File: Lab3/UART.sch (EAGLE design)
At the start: 11 parts, among them IC1 74AC11138, IC2 LM358N, IC3 LM358D, U1 AD558

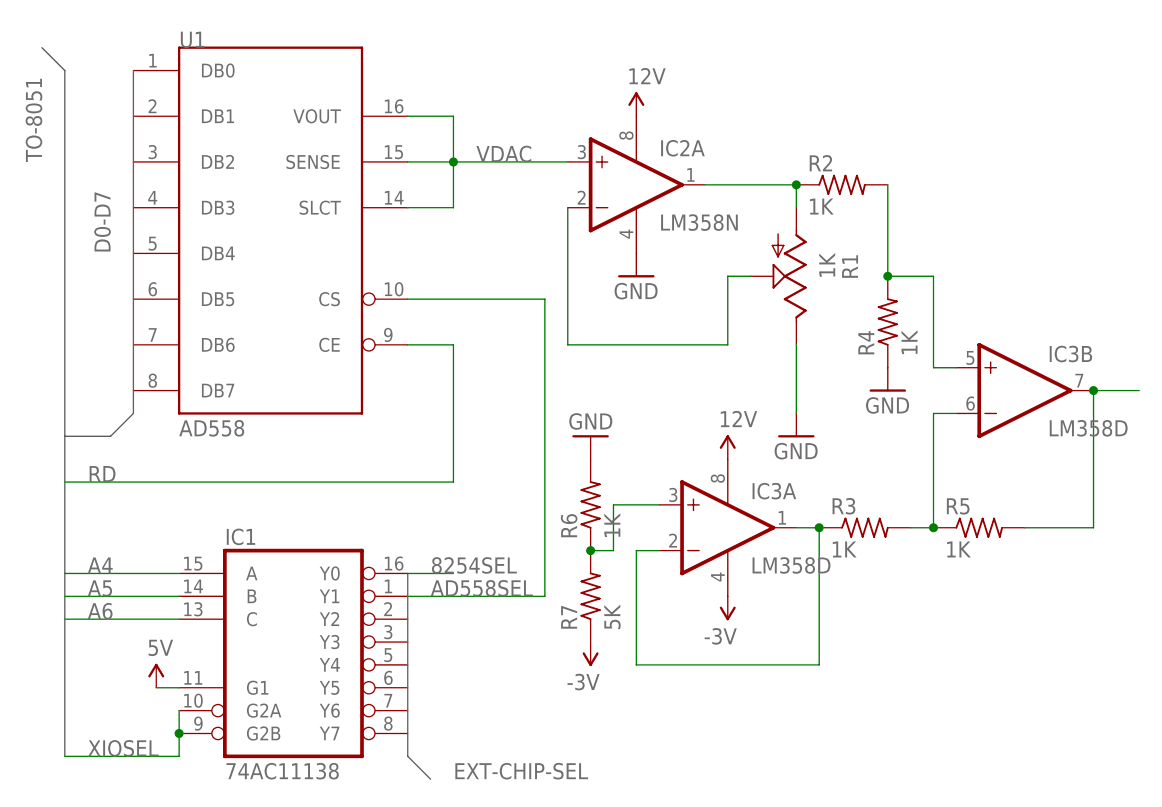
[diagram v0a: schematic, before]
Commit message: halfway through lab 4
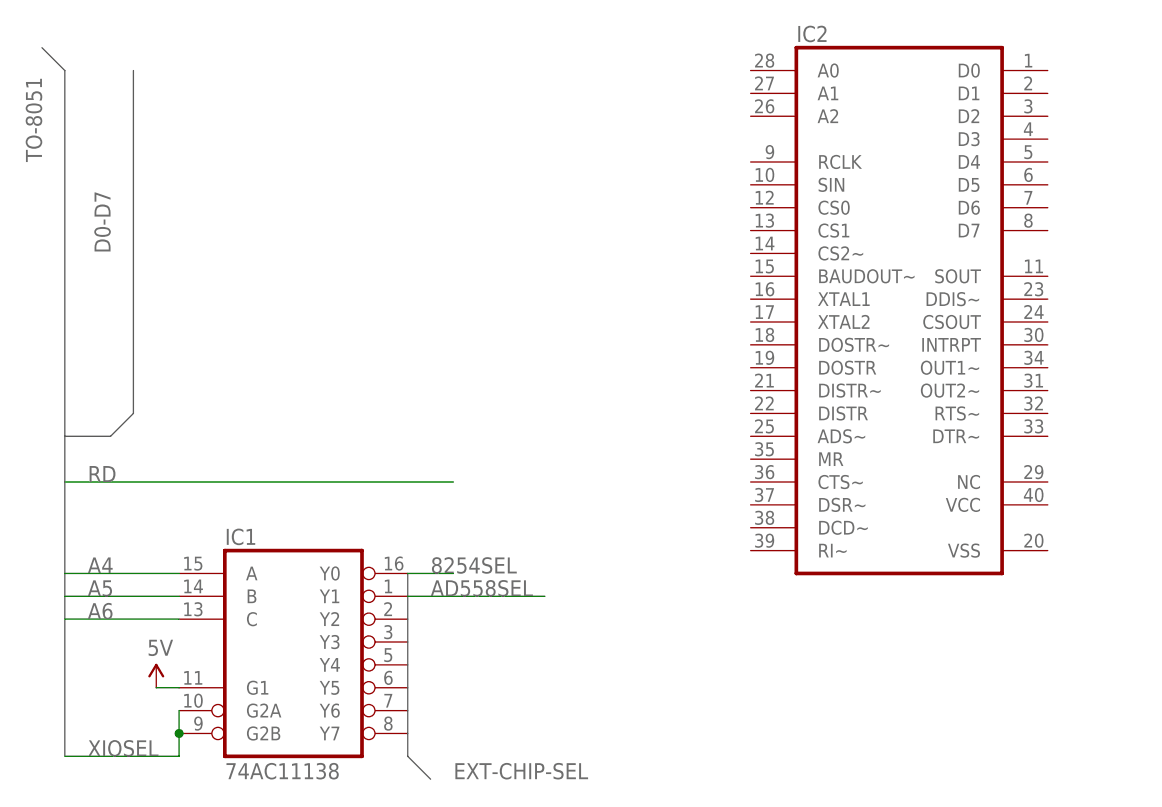
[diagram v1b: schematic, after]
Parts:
- removed IC3: LM358D, linear:LM358D
- removed R1: 1K, pot:TRIM_US-3223G
- removed R2, R3, R4, R5, R6: 1K, resistor:R-US_0204/2V
- removed R7: 5K, resistor:R-US_0204/2V
- removed U1: AD558, AD558:AD558
- IC2: value LM358N -> (none); device linear:LM358N -> exar:XR-16C450P
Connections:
- removed net GND: IC2P.V-, R1.E, R4.1, R6.2
- removed net N$1: IC2A.OUT, R1.A, R2.1
- removed net N$2: IC2A.-IN, R1.S
- removed net N$3: IC3A.-IN, IC3A.OUT, R3.1
- removed net N$4: IC3A.+IN, R6.1, R7.2
- removed net N$5: IC3B.+IN, R2.2, R4.2
- removed net N$6: IC3B.-IN, R3.2, R5.1
- removed net N$8: IC3B.OUT, R5.2
- removed net RD: U1AD558.CE
- removed net VDAC: IC2A.+IN, U1AD558.SENSE, U1AD558.SLCT, U1AD558.VOUT
- net 5V: no longer IC2P.V+, IC3P.V+, IC3P.V-, R7.1
- net AD558SEL: no longer U1AD558.CS
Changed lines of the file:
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@@
 <parts>
 <part name="IC1" library="74ac-logic" deviceset="74AC11138" device=""/>
-<part name="U1" library="AD558" deviceset="AD558" device=""/>
-<part name="IC2" library="linear" deviceset="LM358" device="N"/>
-<part name="R1" library="pot" deviceset="TRIM_US-" device="3223G" value="1K"/>
-<part name="GND1" library="SparkFun-Aesthetics" deviceset="GND" device=""/>
-<part name="SUPPLY1" library="SparkFun-Aesthetics" deviceset="5V" device="" value="12V"/>
 <part name="SUPPLY2" library="SparkFun-Aesthetics" deviceset="5V" device=""/>
-<part name="GND2" library="SparkFun-Aesthetics" deviceset="GND" device=""/>
-<part name="IC3" library="linear" deviceset="LM358" device="D"/>
-<part name="R2" library="resistor" deviceset="R-US_" device="0204/2V" value="1K"/>
-<part name="R3" library="resistor" deviceset="R-US_" device="0204/2V" value="1K"/>
-<part name="R4" library="resistor" deviceset="R-US_" device="0204/2V" value="1K"/>
-<part name="R5" library="resistor" deviceset="R-US_" device="0204/2V" value="1K"/>
-<part name="R6" library="resistor" deviceset="R-US_" device="0204/2V" value="1K"/>
-<part name="R7" library="resistor" deviceset="R-US_" device="0204/2V" value="5K"/>
-<part name="SUPPLY3" library="SparkFun-Aesthetics" deviceset="5V" device="" value="-3V"/>
-<part name="SUPPLY4" library="SparkFun-Aesthetics" deviceset="5V" device="" value="12V"/>
-<part name="SUPPLY5" library="SparkFun-Aesthetics" deviceset="5V" device="" value="-3V"/>
-<part name="GND3" library="SparkFun-Aesthetics" deviceset="GND" device=""/>
-<part name="GND4" library="SparkFun-Aesthetics" deviceset="GND" device=""/>
+<part name="IC2" library="exar" deviceset="XR-16C450P" device=""/>
 </parts>
 <sheets>
@@
 <instances>
 <instance part="IC1" gate="A" x="38.1" y="17.78"/>
-<instance part="U1" gate="AD558" x="33.02" y="63.5"/>
-<instance part="IC2" gate="A" x="73.66" y="68.58"/>
-<instance part="R1" gate="G$1" x="91.44" y="58.42" rot="R180"/>
-<instance part="GND1" gate="1" x="91.44" y="40.64"/>
-<instance part="IC2" gate="P" x="73.66" y="68.58"/>
-<instance part="SUPPLY1" gate="G$1" x="73.66" y="76.2"/>
 <instance part="SUPPLY2" gate="G$1" x="20.32" y="12.7"/>
-<instance part="GND2" gate="1" x="73.66" y="58.42"/>
-<instance part="IC3" gate="A" x="83.82" y="30.48"/>
-<instance part="IC3" gate="B" x="116.84" y="45.72"/>
-<instance part="IC3" gate="P" x="83.82" y="30.48"/>
-<instance part="R2" gate="G$1" x="96.52" y="68.58"/>
-<instance part="R3" gate="G$1" x="99.06" y="30.48"/>
-<instance part="R4" gate="G$1" x="101.6" y="53.34" rot="R90"/>
-<instance part="R5" gate="G$1" x="111.76" y="30.48"/>
-<instance part="R6" gate="G$1" x="68.58" y="33.02" rot="R90"/>
-<instance part="R7" gate="G$1" x="68.58" y="22.86" rot="R90"/>
-<instance part="SUPPLY3" gate="G$1" x="83.82" y="22.86" rot="R180"/>
-<instance part="SUPPLY4" gate="G$1" x="83.82" y="38.1"/>
-<instance part="SUPPLY5" gate="G$1" x="68.58" y="17.78" rot="R180"/>
-<instance part="GND3" gate="1" x="68.58" y="40.64" rot="R180"/>
-<instance part="GND4" gate="1" x="101.6" y="45.72"/>
+<instance part="IC2" gate="G$1" x="101.6" y="55.88"/>
 </instances>
 <busses>
@@
 <pinref part="IC1" gate="A" pin="Y1"/>
 <wire x1="48.26" y1="22.86" x2="63.5" y2="22.86" width="0.1524" layer="91"/>
-<wire x1="63.5" y1="22.86" x2="63.5" y2="55.88" width="0.1524" layer="91"/>
-<pinref part="U1" gate="AD558" pin="CS"/>
-<wire x1="48.26" y1="55.88" x2="63.5" y2="55.88" width="0.1524" layer="91"/>
 <label x="50.8" y="22.86" size="1.778" layer="95"/>
 </segment>
@@
 <net name="RD" class="0">
 <segment>
-<pinref part="U1" gate="AD558" pin="CE"/>
-<wire x1="48.26" y1="50.8" x2="53.34" y2="50.8" width="0.1524" layer="91"/>
 <label x="12.7" y="35.56" size="1.778" layer="95"/>
-<wire x1="53.34" y1="50.8" x2="53.34" y2="35.56" width="0.1524" layer="91"/>
 <wire x1="53.34" y1="35.56" x2="10.16" y2="35.56" width="0.1524" layer="91"/>
-</segment>
-</net>
-<net name="VDAC" class="0">
-<segment>
-<pinref part="U1" gate="AD558" pin="VOUT"/>
-<wire x1="48.26" y1="76.2" x2="53.34" y2="76.2" width="0.1524" layer="91"/>
-<pinref part="U1" gate="AD558" pin="SENSE"/>
-<wire x1="48.26" y1="71.12" x2="53.34" y2="71.12" width="0.1524" layer="91"/>
-<wire x1="53.34" y1="71.12" x2="53.34" y2="76.2" width="0.1524" layer="91"/>
-<pinref part="U1" gate="AD558" pin="SLCT"/>
-<wire x1="48.26" y1="66.04" x2="53.34" y2="66.04" width="0.1524" layer="91"/>
-<wire x1="53.34" y1="66.04" x2="53.34" y2="71.12" width="0.1524" layer="91"/>
-<junction x="53.34" y="71.12"/>
-<label x="55.88" y="71.12" size="1.778" layer="95"/>
-<pinref part="IC2" gate="A" pin="+IN"/>
-<wire x1="53.34" y1="71.12" x2="66.04" y2="71.12" width="0.1524" layer="91"/>
 </segment>
 </net>
@@
 </segment>
 </net>
-<net name="N$2" class="0">
-<segment>
-<pinref part="IC2" gate="A" pin="-IN"/>
-<wire x1="66.04" y1="66.04" x2="66.04" y2="50.8" width="0.1524" layer="91"/>
-<wire x1="66.04" y1="50.8" x2="83.82" y2="50.8" width="0.1524" layer="91"/>
-<wire x1="83.82" y1="50.8" x2="83.82" y2="58.42" width="0.1524" layer="91"/>
-<pinref part="R1" gate="G$1" pin="S"/>
-<wire x1="83.82" y1="58.42" x2="86.36" y2="58.42" width="0.1524" layer="91"/>
-</segment>
-</net>
-<net name="GND" class="0">
-<segment>
-<pinref part="R1" gate="G$1" pin="E"/>
-<pinref part="GND1" gate="1" pin="GND"/>
-<wire x1="91.44" y1="50.8" x2="91.44" y2="43.18" width="0.1524" layer="91"/>
-</segment>
-<segment>
-<pinref part="IC2" gate="P" pin="V-"/>
-<pinref part="GND2" gate="1" pin="GND"/>
-</segment>
-<segment>
-<pinref part="R6" gate="G$1" pin="2"/>
-<pinref part="GND3" gate="1" pin="GND"/>
-</segment>
-<segment>
-<pinref part="R4" gate="G$1" pin="1"/>
-<pinref part="GND4" gate="1" pin="GND"/>
-</segment>
-</net>
 <net name="5V" class="0">
 <segment>
@@
 <pinref part="SUPPLY2" gate="G$1" pin="5V"/>
 </segment>
-<segment>
-<pinref part="SUPPLY1" gate="G$1" pin="5V"/>
-<pinref part="IC2" gate="P" pin="V+"/>
-</segment>
-<segment>
-<pinref part="IC3" gate="P" pin="V-"/>
-<pinref part="SUPPLY3" gate="G$1" pin="5V"/>
-</segment>
-<segment>
-<pinref part="IC3" gate="P" pin="V+"/>
-<pinref part="SUPPLY4" gate="G$1" pin="5V"/>
-</segment>
-<segment>
-<pinref part="R7" gate="G$1" pin="1"/>
-<pinref part="SUPPLY5" gate="G$1" pin="5V"/>
-</segment>
 </net>
-<net name="N$1" class="0">
-<segment>
-<pinref part="IC2" gate="A" pin="OUT"/>
-<wire x1="81.28" y1="68.58" x2="91.44" y2="68.58" width="0.1524" layer="91"/>
-<pinref part="R1" gate="G$1" pin="A"/>
-<wire x1="91.44" y1="68.58" x2="91.44" y2="66.04" width="0.1524" layer="91"/>
-<pinref part="R2" gate="G$1" pin="1"/>
-<junction x="91.44" y="68.58"/>
-</segment>
-</net>
-<net name="N$3" class="0">
-<segment>
-<pinref part="IC3" gate="A" pin="-IN"/>
-<wire x1="76.2" y1="27.94" x2="73.66" y2="27.94" width="0.1524" layer="91"/>
-<wire x1="73.66" y1="27.94" x2="73.66" y2="15.24" width="0.1524" layer="91"/>
-<pinref part="IC3" gate="A" pin="OUT"/>
-<wire x1="93.98" y1="30.48" x2="91.44" y2="30.48" width="0.1524" layer="91"/>
-<wire x1="73.66" y1="15.24" x2="93.98" y2="15.24" width="0.1524" layer="91"/>
-<wire x1="93.98" y1="15.24" x2="93.98" y2="30.48" width="0.1524" layer="91"/>
-<pinref part="R3" gate="G$1" pin="1"/>
-<junction x="93.98" y="30.48"/>
-</segment>
-</net>
-<net name="N$4" class="0">
-<segment>
-<pinref part="R7" gate="G$1" pin="2"/>
-<pinref part="R6" gate="G$1" pin="1"/>
-<wire x1="68.58" y1="27.94" x2="71.12" y2="27.94" width="0.1524" layer="91"/>
-<wire x1="71.12" y1="27.94" x2="71.12" y2="33.02" width="0.1524" layer="91"/>
-<junction x="68.58" y="27.94"/>
-<pinref part="IC3" gate="A" pin="+IN"/>
-<wire x1="71.12" y1="33.02" x2="76.2" y2="33.02" width="0.1524" layer="91"/>
-</segment>
-</net>
-<net name="N$5" class="0">
-<segment>
-<pinref part="R2" gate="G$1" pin="2"/>
-<pinref part="R4" gate="G$1" pin="2"/>
-<wire x1="101.6" y1="58.42" x2="101.6" y2="68.58" width="0.1524" layer="91"/>
-<wire x1="101.6" y1="58.42" x2="106.68" y2="58.42" width="0.1524" layer="91"/>
-<wire x1="106.68" y1="58.42" x2="106.68" y2="48.26" width="0.1524" layer="91"/>
-<junction x="101.6" y="58.42"/>
-<pinref part="IC3" gate="B" pin="+IN"/>
-<wire x1="106.68" y1="48.26" x2="109.22" y2="48.26" width="0.1524" layer="91"/>
-</segment>
-</net>
-<net name="N$6" class="0">
-<segment>
-<pinref part="R3" gate="G$1" pin="2"/>
-<pinref part="R5" gate="G$1" pin="1"/>
-<pinref part="IC3" gate="B" pin="-IN"/>
-<wire x1="109.22" y1="43.18" x2="106.68" y2="43.18" width="0.1524" layer="91"/>
-<wire x1="106.68" y1="43.18" x2="106.68" y2="30.48" width="0.1524" layer="91"/>
-<junction x="106.68" y="30.48"/>
-<wire x1="106.68" y1="30.48" x2="104.14" y2="30.48" width="0.1524" layer="91"/>
-</segment>
-</net>
-<net name="N$8" class="0">
-<segment>
-<pinref part="IC3" gate="B" pin="OUT"/>
-<wire x1="124.46" y1="45.72" x2="124.46" y2="30.48" width="0.1524" layer="91"/>
-<pinref part="R5" gate="G$1" pin="2"/>
-<wire x1="124.46" y1="30.48" x2="116.84" y2="30.48" width="0.1524" layer="91"/>
-<wire x1="124.46" y1="45.72" x2="129.54" y2="45.72" width="0.1524" layer="91"/>
-<junction x="124.46" y="45.72"/>
-</segment>
-</net>
